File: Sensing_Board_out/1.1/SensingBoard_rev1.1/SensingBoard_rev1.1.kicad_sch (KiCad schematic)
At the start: 89 parts, among them J1 USB_C_Receptacle, J3 F32R-1A7H1-11024, J5 RS1-02-G, J6 RS1-02-G, J7 3221-10-0300-00, J7 RS1-02-G, J9 RS1-02-G, SW1 PTS815 SJM 250 SMTR LFS, SW2 PTS815 SJM 250 SMTR LFS, U2 BNO055, U3 MIC5504-3.3YM5, U4 FT232RQ, U5 MIC5504-1.8YM5, U6 MCP1700x-280xxTT, U7 ESP32-S3, U8 GD25D05CT, Y1 ABM8G-40.000MHZ-18-D2Y-T

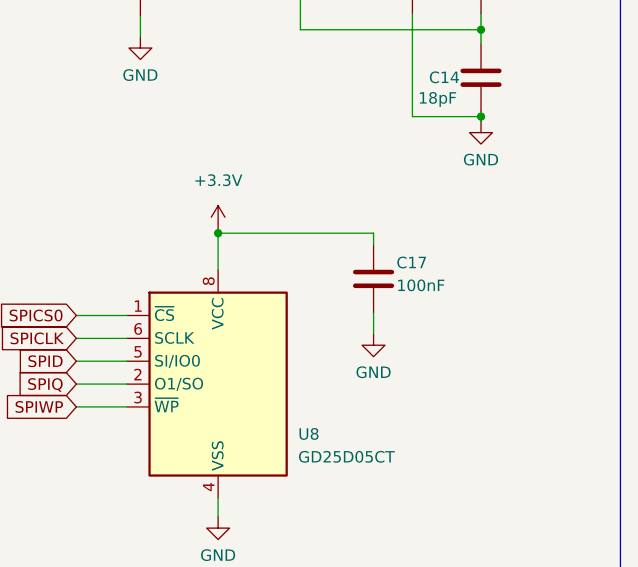
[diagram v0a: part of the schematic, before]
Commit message: power board layout
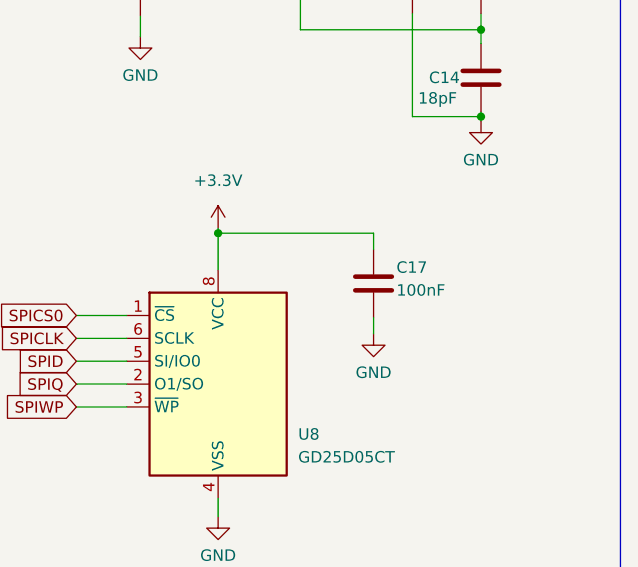
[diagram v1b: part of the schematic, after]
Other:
- moved on the sheet: C17
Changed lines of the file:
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@@
     (stroke (width 0) (type default))
   )
-  (wire (pts (xy 541.274 243.586) (xy 541.274 241.3))
+  (wire (pts (xy 541.274 243.586) (xy 541.274 241.808))
     (stroke (width 0) (type default))
   )
@@
     (stroke (width 0) (type default))
   )
-  (wire (pts (xy 541.274 233.68) (xy 541.274 232.41))
+  (wire (pts (xy 541.274 234.188) (xy 541.274 232.41))
     (stroke (width 0) (type default))
   )
@@
     )
   )
-  (symbol (lib_id "Device:C") (at 541.274 237.49 0) (unit 1)
+  (symbol (lib_id "Device:C") (at 541.274 237.998 0) (unit 1)
     (in_bom yes) (on_board yes) (dnp no)
-    (property "Reference" "C17" (at 543.814 235.712 0)
+    (property "Reference" "C17" (at 543.814 236.22 0)
       (effects (font (size 1.27 1.27)) (justify left))
     )
-    (property "Value" "100nF" (at 543.814 238.252 0)
+    (property "Value" "100nF" (at 543.814 238.76 0)
       (effects (font (size 1.27 1.27)) (justify left))
     )
-    (property "Footprint" "Capacitor_SMD:C_0402_1005Metric" (at 542.2392 241.3 0)
+    (property "Footprint" "Capacitor_SMD:C_0402_1005Metric" (at 542.2392 241.808 0)
       (effects (font (size 1.27 1.27)) hide)
     )
-    (property "Datasheet" "~" (at 541.274 237.49 0)
+    (property "Datasheet" "~" (at 541.274 237.998 0)
       (effects (font (size 1.27 1.27)) hide)
     )

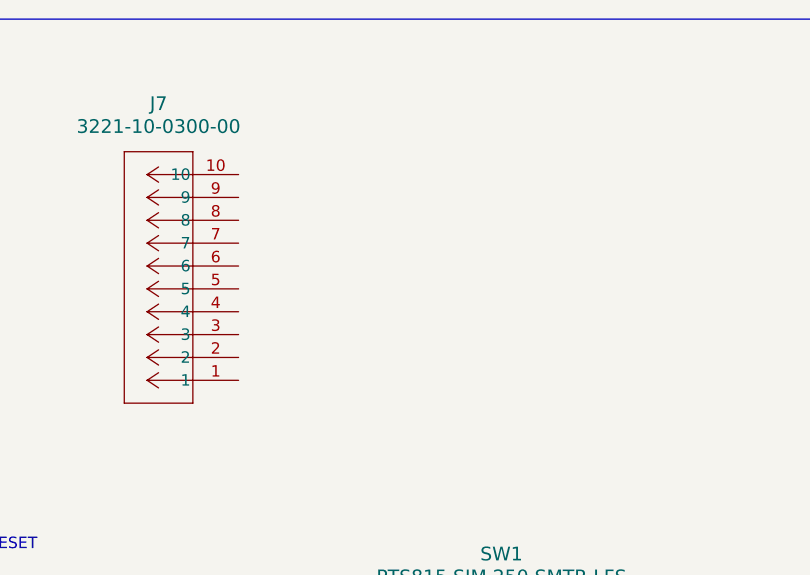
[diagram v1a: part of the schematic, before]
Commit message: checking drc
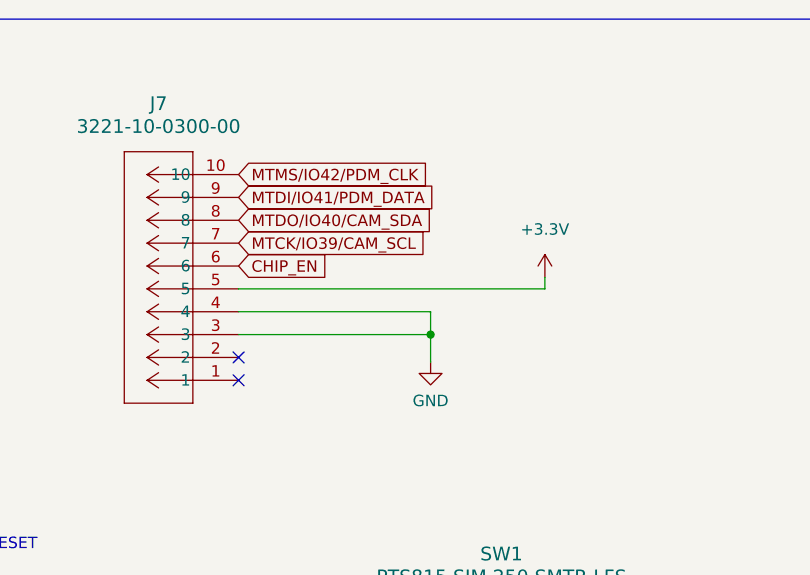
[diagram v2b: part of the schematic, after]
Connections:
- net +3.3V: now also J7.5
- net CHIP_EN: now also J7.6
- net GND: now also J7.3, J7.4
- net MTCK/IO39/CAM_SCL: now also J7.7
- net MTDI/IO41/PDM_DATA: now also J7.9
- net MTDO/IO40/CAM_SDA: now also J7.8
- net MTMS/IO42/PDM_CLK: now also J7.10
- no-connect marks 10 -> 12
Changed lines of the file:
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@@
   (junction (at 534.162 175.514) (diameter 0) (color 0 0 0 0)
   )
+  (junction (at 198.374 313.944) (diameter 0) (color 0 0 0 0)
+  )
   (junction (at 187.198 52.324) (diameter 0) (color 0 0 0 0)
   )
@@
   )
   (no_connect (at 69.596 167.386))
+  (no_connect (at 177.038 319.024))
+  (no_connect (at 177.038 316.484))
   (no_connect (at 69.596 180.086))
   (no_connect (at 69.596 182.626))
@@
     (stroke (width 0) (type default))
   )
+  (wire (pts (xy 211.074 308.864) (xy 211.074 307.594))
+    (stroke (width 0) (type default))
+  )
   (wire (pts (xy 337.82 329.946) (xy 357.378 329.946))
     (stroke (width 0) (type default))
@@
     (stroke (width 0) (type default))
   )
+  (wire (pts (xy 198.374 313.944) (xy 198.374 316.992))
+    (stroke (width 0) (type default))
+  )
   (wire (pts (xy 511.302 199.39) (xy 515.366 199.39))
     (stroke (width 0) (type default))
@@
     (stroke (width 0) (type default))
   )
+  (wire (pts (xy 177.038 313.944) (xy 198.374 313.944))
+    (stroke (width 0) (type default))
+  )
   (wire (pts (xy 358.394 213.36) (xy 358.394 215.392))
     (stroke (width 0) (type default))
@@
     (stroke (width 0) (type default))
   )
+  (wire (pts (xy 177.038 308.864) (xy 211.074 308.864))
+    (stroke (width 0) (type default))
+  )
   (wire (pts (xy 49.53 340.614) (xy 49.53 341.884))
     (stroke (width 0) (type default))
@@
     (stroke (width 0) (type default))
   )
+  (wire (pts (xy 198.374 311.404) (xy 198.374 313.944))
+    (stroke (width 0) (type default))
+  )
   (wire (pts (xy 477.52 205.232) (xy 469.646 205.232))
     (stroke (width 0) (type default))
   )
+  (wire (pts (xy 177.038 311.404) (xy 198.374 311.404))
+    (stroke (width 0) (type default))
+  )
   (wire (pts (xy 164.084 345.44) (xy 165.608 345.44))
     (stroke (width 0) (type default))
@@
     )
   )
+  (global_label "MTDI{slash}IO41{slash}PDM_DATA" (shape input) (at 177.038 298.704 0) (fields_autoplaced)
+    (effects (font (size 1.27 1.27)) (justify left))
+    (property "Intersheetrefs" "${INTERSHEET_REFS}" (at 200.7061 298.704 0)
+      (effects (font (size 1.27 1.27)) (justify left) hide)
+    )
+  )
   (global_label "SPIWP" (shape input) (at 477.266 233.172 0) (fields_autoplaced)
     (effects (font (size 1.27 1.27)) (justify left))
@@
     )
   )
+  (global_label "MTDO{slash}IO40{slash}CAM_SDA" (shape input) (at 177.038 301.244 0) (fields_autoplaced)
+    (effects (font (size 1.27 1.27)) (justify left))
+    (property "Intersheetrefs" "${INTERSHEET_REFS}" (at 200.4037 301.244 0)
+      (effects (font (size 1.27 1.27)) (justify left) hide)
+    )
+  )
   (global_label "IO18{slash}DVP_Y4" (shape input) (at 83.312 298.45 180) (fields_autoplaced)
     (effects (font (size 1.27 1.27)) (justify right))
@@
     )
   )
+  (global_label "MTCK{slash}IO39{slash}CAM_SCL" (shape input) (at 177.038 303.784 0) (fields_autoplaced)
+    (effects (font (size 1.27 1.27)) (justify left))
+    (property "Intersheetrefs" "${INTERSHEET_REFS}" (at 200.2827 303.784 0)
+      (effects (font (size 1.27 1.27)) (justify left) hide)
+    )
+  )
   (global_label "IO11{slash}DVP_Y8" (shape input) (at 84.074 278.13 180) (fields_autoplaced)
     (effects (font (size 1.27 1.27)) (justify right))
@@
     )
   )
+  (global_label "CHIP_EN" (shape input) (at 177.038 306.324 0) (fields_autoplaced)
+    (effects (font (size 1.27 1.27)) (justify left))
+    (property "Intersheetrefs" "${INTERSHEET_REFS}" (at 187.9456 306.324 0)
+      (effects (font (size 1.27 1.27)) (justify left) hide)
+    )
+  )
   (global_label "SPICLK" (shape input) (at 508.254 244.094 180) (fields_autoplaced)
     (effects (font (size 1.27 1.27)) (justify right))
@@
     )
   )
+  (global_label "MTMS{slash}IO42{slash}PDM_CLK" (shape input) (at 177.038 296.164 0) (fields_autoplaced)
+    (effects (font (size 1.27 1.27)) (justify left))
+    (property "Intersheetrefs" "${INTERSHEET_REFS}" (at 200.6455 296.164 0)
+      (effects (font (size 1.27 1.27)) (justify left) hide)
+    )
+  )
   (global_label "GPIO33" (shape input) (at 405.384 332.486 0) (fields_autoplaced)
     (effects (font (size 1.27 1.27)) (justify left))
@@
     )
   )
+  (symbol (lib_id "power:GND") (at 198.374 316.992 0) (unit 1)
+    (in_bom yes) (on_board yes) (dnp no) (fields_autoplaced)
+    (property "Reference" "#PWR069" (at 198.374 323.342 0)
+      (effects (font (size 1.27 1.27)) hide)
+    )
+    (property "Value" "GND" (at 198.374 321.31 0)
+      (effects (font (size 1.27 1.27)))
+    )
+    (property "Footprint" "" (at 198.374 316.992 0)
+      (effects (font (size 1.27 1.27)) hide)
+    )
+    (property "Datasheet" "" (at 198.374 316.992 0)
+      (effects (font (size 1.27 1.27)) hide)
+    )
+    (pin "1")
+    (instances
+      (project "SensingBoard_rev1.1"
+        (path "/b61d80ec-963d-4516-bd15-8e7f6f5207da"
+          (reference "#PWR069") (unit 1)
+        )
+      )
+    )
+  )
   (symbol (lib_id "ABM8G_40_000MHZ_18_D2Y_T:ABM8G-40.000MHZ-18-D2Y-T") (at 553.212 208.026 270) (mirror x) (unit 1)
     (in_bom yes) (on_board yes) (dnp no)
@@
         )
       )
+    )
+  )
+  (symbol (lib_id "power:+3.3V") (at 211.074 307.594 0) (unit 1)
+    (in_bom yes) (on_board yes) (dnp no)
+    (property "Reference" "#PWR068" (at 211.074 311.404 0)
+      (effects (font (size 1.27 1.27)) hide)
+    )
+    (property "Value" "+3.3V" (at 211.074 302.26 0)
+      (effects (font (size 1.27 1.27)))
+    )
+    (property "Footprint" "" (at 211.074 307.594 0)
+      (effects (font (size 1.27 1.27)) hide)
+    )
+    (property "Datasheet" "" (at 211.074 307.594 0)
+      (effects (font (size 1.27 1.27)) hide)
+    )
+    (pin "1")
+    (instances
+      (project "SensingBoard_rev1.1"
+        (path "/b61d80ec-963d-4516-bd15-8e7f6f5207da"
+          (reference "#PWR068") (unit 1)
+        )
+      )
